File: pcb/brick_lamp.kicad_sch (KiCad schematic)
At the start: 11 parts, among them J1 LED_24V_OUT, J2 24V_IN, J3 DEBUG, J4 DEBUG, Q1 CSD17302Q5A, U2 MCP1799x-330xxTT, U3 ATtiny85V-10S

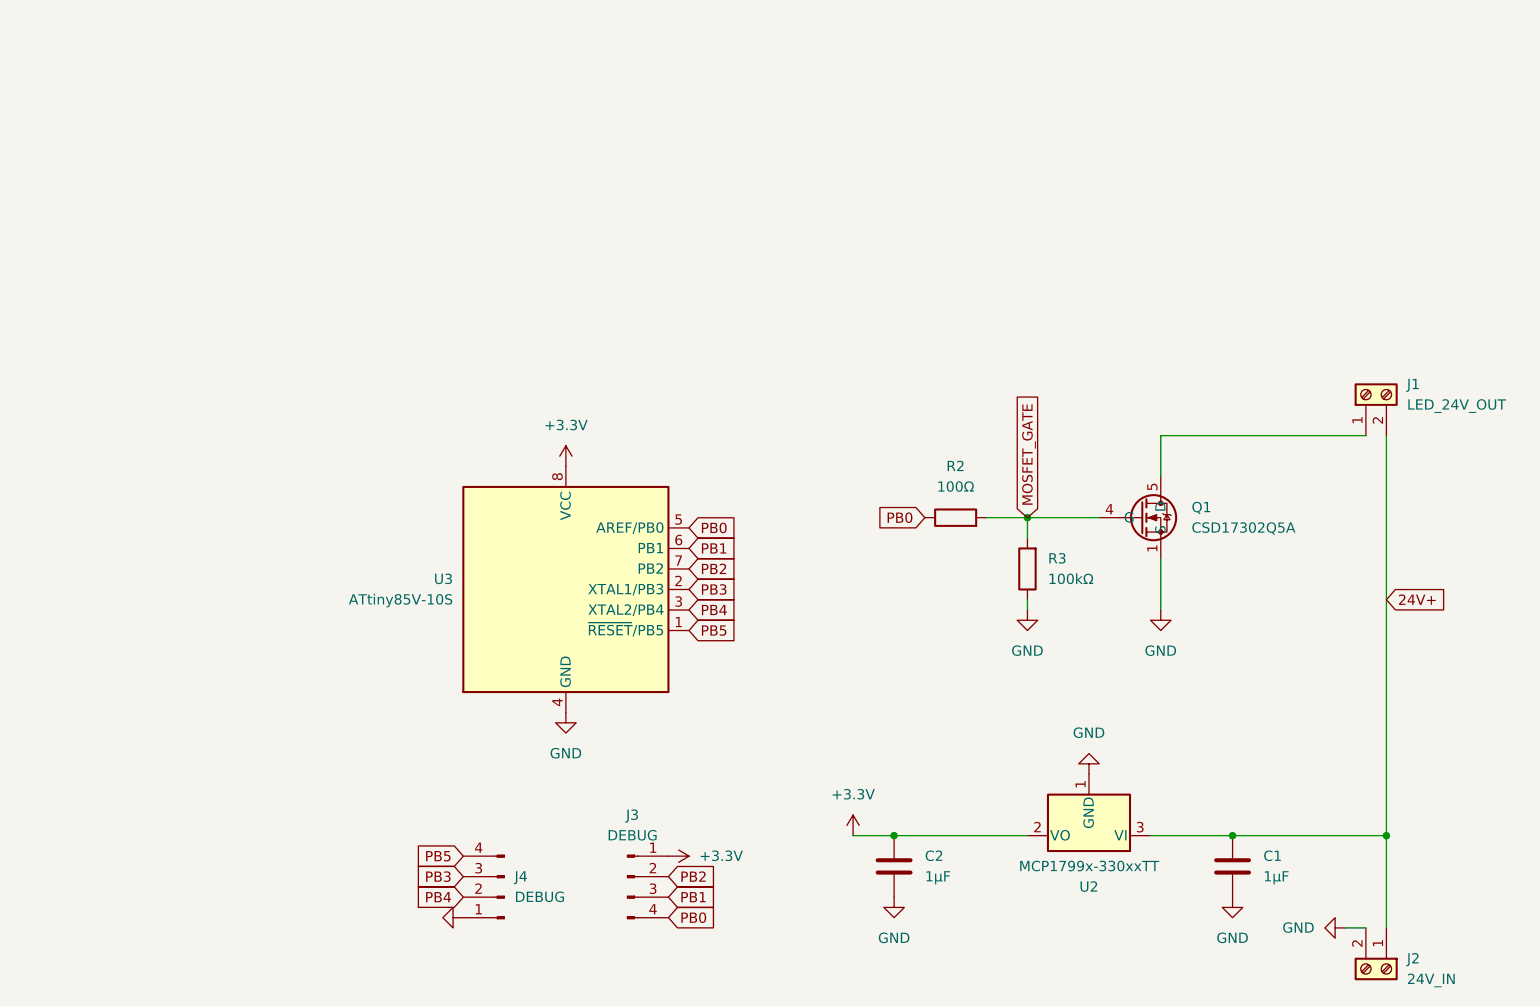
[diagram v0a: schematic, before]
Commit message: Cleanup the layout and schematic
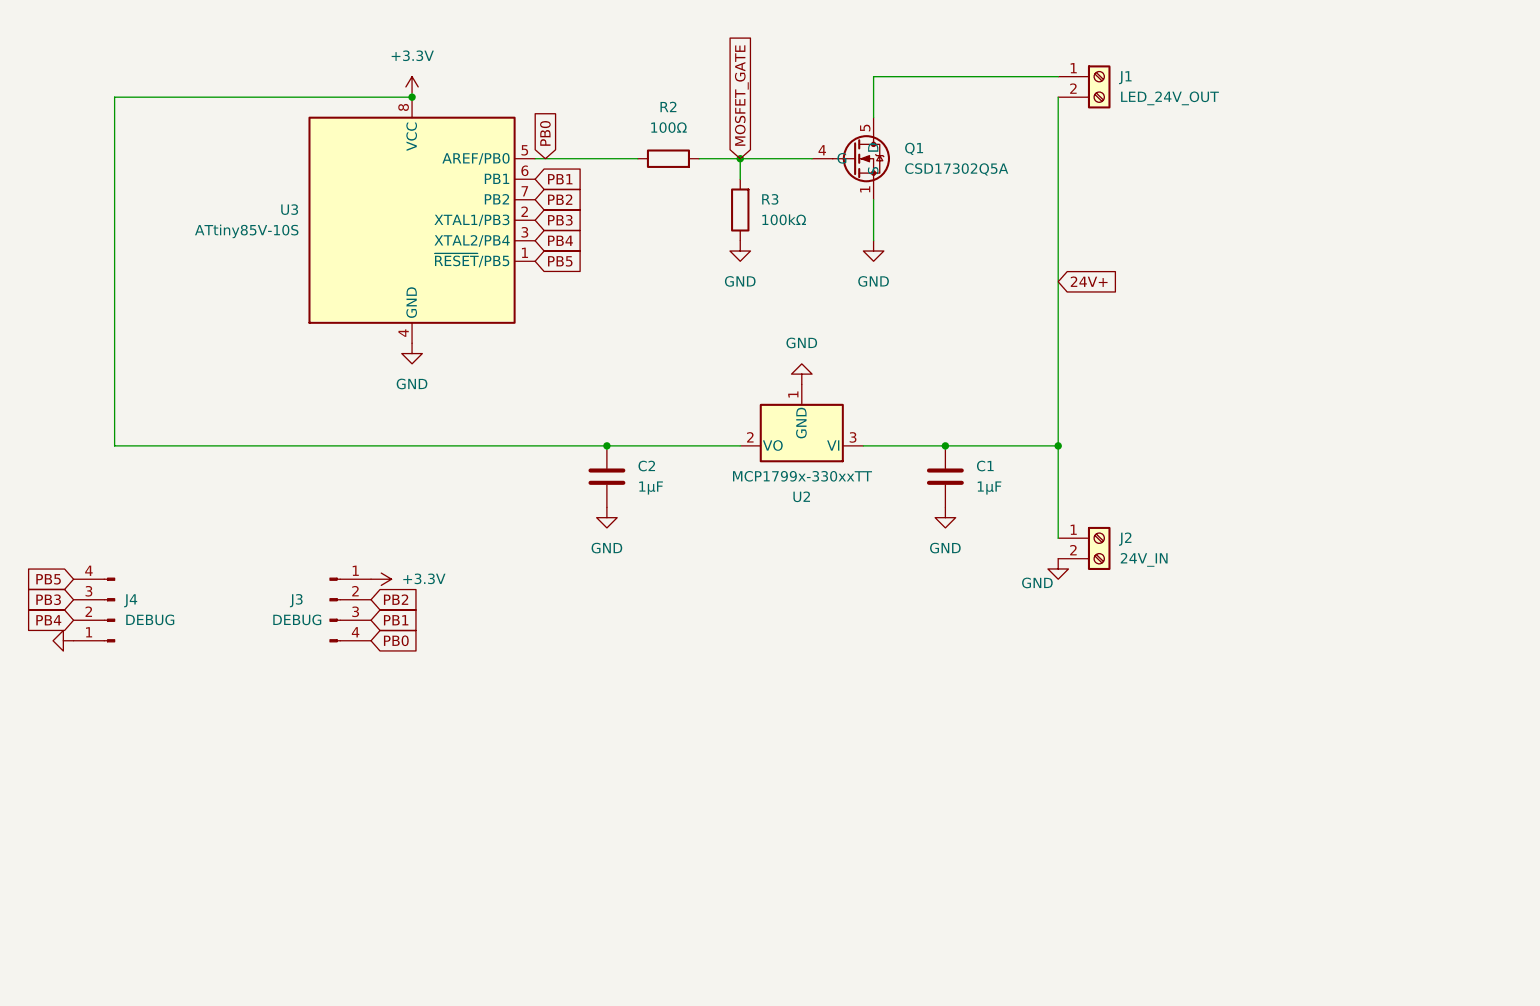
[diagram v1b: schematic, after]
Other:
- moved on the sheet: C1, C2, J1, J2, J3, J4, Q1, R2, R3, U2, U3
